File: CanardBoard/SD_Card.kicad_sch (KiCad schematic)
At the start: 9 parts, among them J1 Conn_ST_STDC14, J2 Micro_SD_Card, J4 USB_C_Receptacle_USB2.0_16P

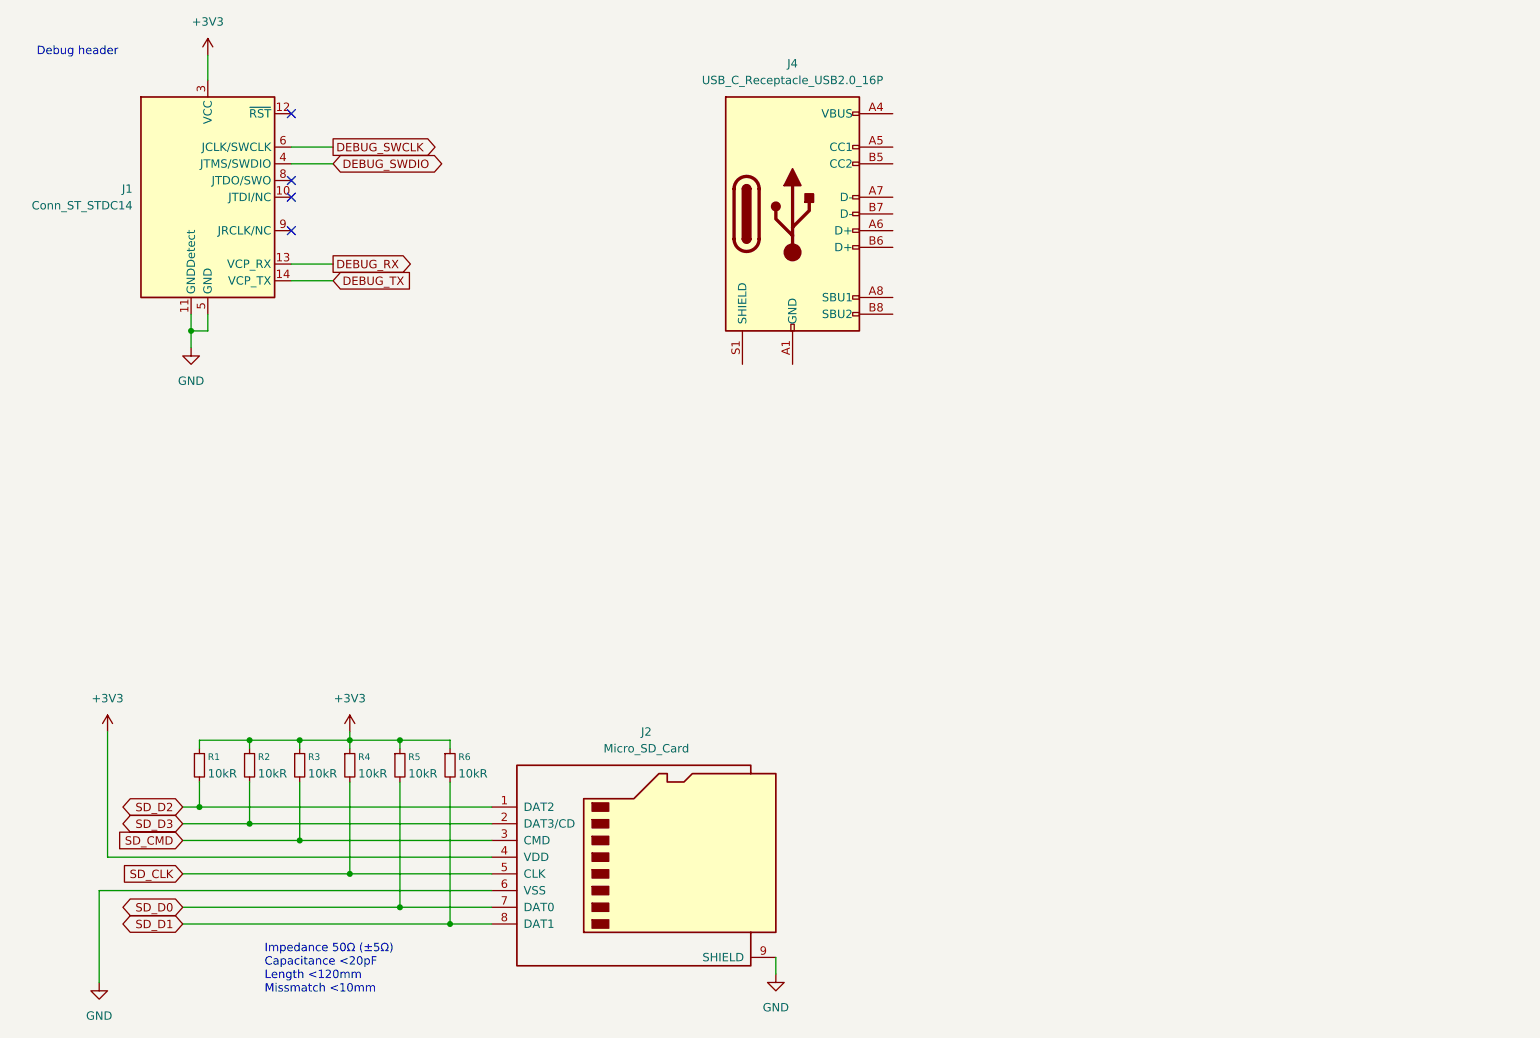
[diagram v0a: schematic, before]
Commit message: schematic work
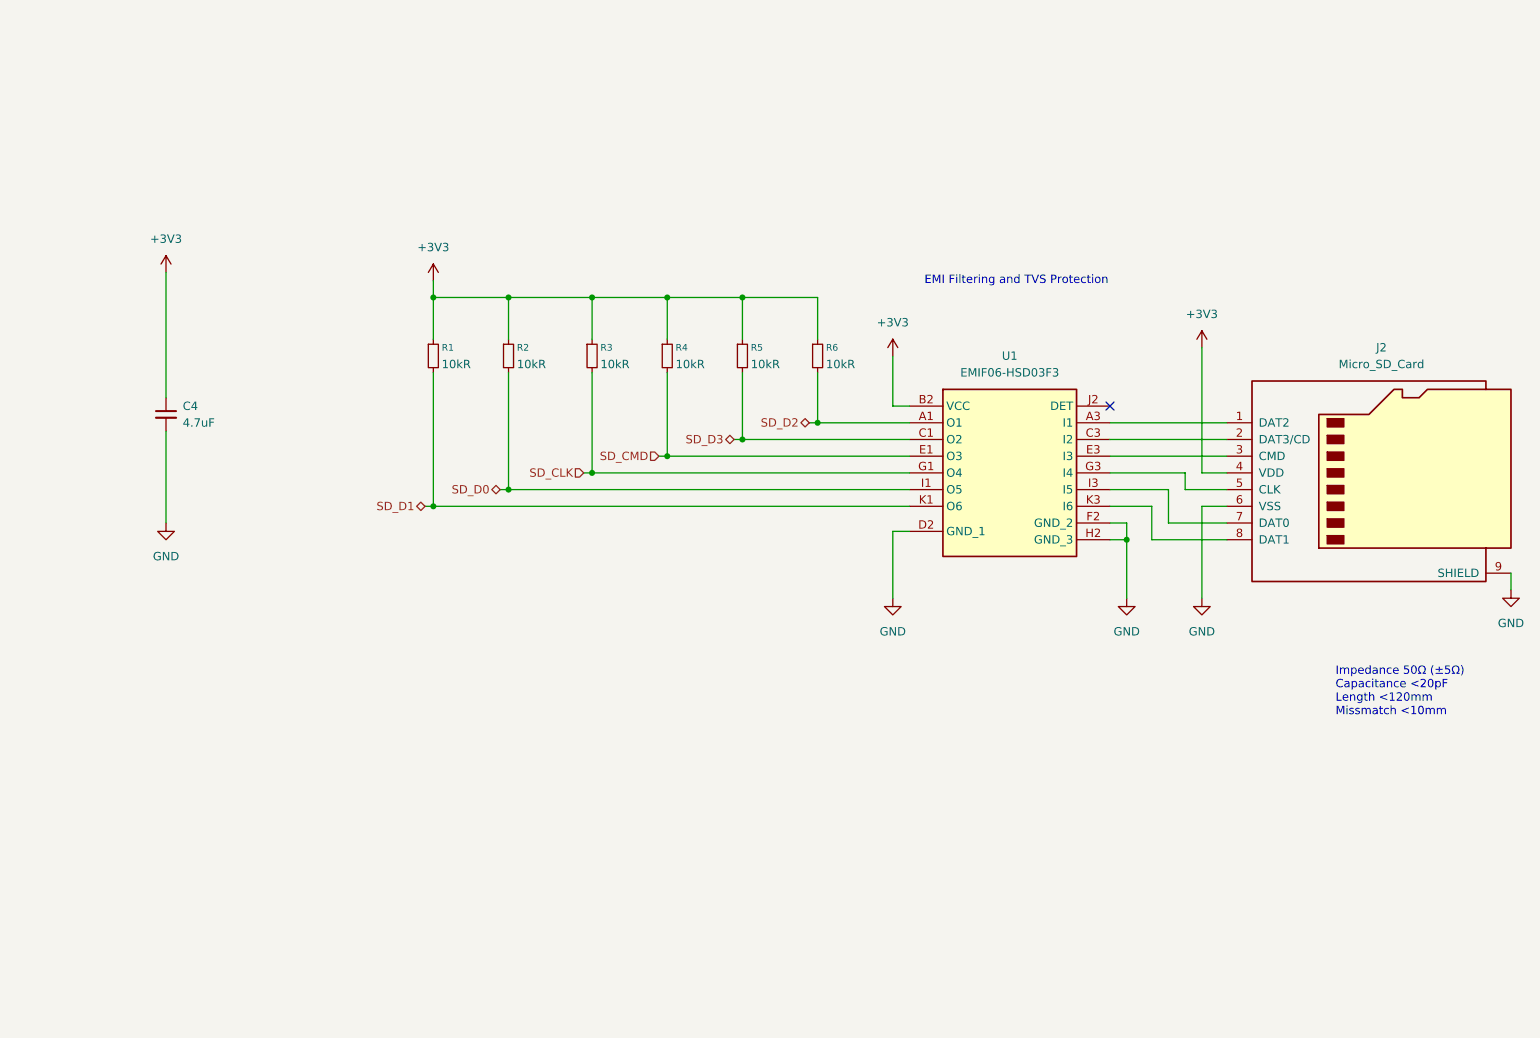
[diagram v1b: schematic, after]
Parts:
- removed J1: Conn_ST_STDC14, Connector_PinHeader_1.27mm:PinHeader_2x07_P1.27mm_Vertical, symbol Connector:Conn_ST_STDC14
- removed J4: USB_C_Receptacle_USB2.0_16P, Connector_USB:USB_C_Receptacle_GCT_USB4105-xx-A_16P_TopMnt_Horizontal, symbol Connector:USB_C_Receptacle_USB2.0_16P
- added C4: 4.7uF, Capacitor_SMD:C_0805_2012Metric_Pad1.18x1.45mm_HandSolder, symbol Device_Custom:C_Small
- added U1: EMIF06-HSD03F3, EMIF06HSD03F3, symbol canhw:EMIF06-HSD03F3
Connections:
- net +3V3: now also C4.1, U1.B2 (VCC)
- net GND: now also C4.2, U1.D2 (GND_1), U1.F2 (GND_2), U1.H2 (GND_3)
- net SD_CLK: now also R3.2, U1.G1 (O4); no longer J2.5 (CLK), R4.2
- net SD_CMD: now also R4.2, U1.E1 (O3); no longer J2.3 (CMD), R3.2
- net SD_D0: now also R2.2, U1.I1 (O5); no longer J2.7 (DAT0), R5.2
- net SD_D1: now also R1.2, U1.K1 (O6); no longer J2.8 (DAT1), R6.2
- net SD_D2: now also R6.2, U1.A1 (O1); no longer J2.1 (DAT2), R1.2
- net SD_D3: now also R5.2, U1.C1 (O2); no longer J2.2 (DAT3/CD), R2.2
- new net: J2.1 (DAT2), U1.A3 (I1)
- new net: J2.2 (DAT3/CD), U1.C3 (I2)
- new net: J2.3 (CMD), U1.E3 (I3)
- new net: J2.5 (CLK), U1.G3 (I4)
- new net: J2.7 (DAT0), U1.I3 (I5)
- new net: J2.8 (DAT1), U1.K3 (I6)
- no-connect marks 4 -> 1
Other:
- note added: "EMI Filtering and TVS Protection"
- note removed: "Debug header"
- moved on the sheet: J2, R1, R2, R3, R4, R5, R6

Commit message: make project symbols and footprints
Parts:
- U1: symbol canhw:EMIF06-HSD03F3 -> canardboard:EMIF06-HSD03F3
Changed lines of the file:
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@@
 	)
 	(symbol
-		(lib_id "canhw:EMIF06-HSD03F3")
+		(lib_id "canardboard:EMIF06-HSD03F3")
 		(at 165.1 87.63 0)
 		(unit 1)

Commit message: work
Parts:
- C4: footprint Capacitor_SMD:C_0805_2012Metric_Pad1.18x1.45mm_HandSolder -> Capacitor_SMD:C_0402_1005Metric
- R1, R2, R3, R4, R5, R6: footprint Resistor_SMD:R_0201_0603Metric -> Resistor_SMD:R_0402_1005Metric
- U1: footprint EMIF06HSD03F3 -> canardboard:EMIF06HSD03F3
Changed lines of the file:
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@@
 			)
 		)
-		(property "Footprint" "Capacitor_SMD:C_0805_2012Metric_Pad1.18x1.45mm_HandSolder"
+		(property "Footprint" "Capacitor_SMD:C_0402_1005Metric"
 			(at 52.07 88.9 0)
 			(effects
@@
 			)
 		)
-		(property "Footprint" "Resistor_SMD:R_0201_0603Metric"
+		(property "Footprint" "Resistor_SMD:R_0402_1005Metric"
 			(at 92.71 80.01 0)
 			(effects
@@
 			)
 		)
-		(property "Footprint" "Resistor_SMD:R_0201_0603Metric"
+		(property "Footprint" "Resistor_SMD:R_0402_1005Metric"
 			(at 139.7 80.01 0)
 			(effects
@@
 			)
 		)
-		(property "Footprint" "Resistor_SMD:R_0201_0603Metric"
+		(property "Footprint" "Resistor_SMD:R_0402_1005Metric"
 			(at 128.27 80.01 0)
 			(effects
@@
 			)
 		)
-		(property "Footprint" "EMIF06HSD03F3"
+		(property "Footprint" "canardboard:EMIF06HSD03F3"
 			(at 191.77 182.55 0)
 			(effects
@@
 			)
 		)
-		(property "Footprint" "Resistor_SMD:R_0201_0603Metric"
+		(property "Footprint" "Resistor_SMD:R_0402_1005Metric"
 			(at 104.14 80.01 0)
 			(effects
@@
 			)
 		)
-		(property "Footprint" "Resistor_SMD:R_0201_0603Metric"
+		(property "Footprint" "Resistor_SMD:R_0402_1005Metric"
 			(at 151.13 80.01 0)
 			(effects
@@
 			)
 		)
-		(property "Footprint" "Resistor_SMD:R_0201_0603Metric"
+		(property "Footprint" "Resistor_SMD:R_0402_1005Metric"
 			(at 116.84 80.01 0)
 			(effects
